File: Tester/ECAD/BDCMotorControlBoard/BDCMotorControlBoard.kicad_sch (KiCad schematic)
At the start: 45 parts, among them J3 SWIM connector, J4 Power connector, J5 Motor connector, J6 RS485 connector, Q1 2N7002, Q2 2N7002, Q7 2N7002, Q8 2N7002, SW1 SW_Push, U1 STM8S003F3P6, U3 SP485, U4 L78M05_TO252, Y1 Crystal_GND24

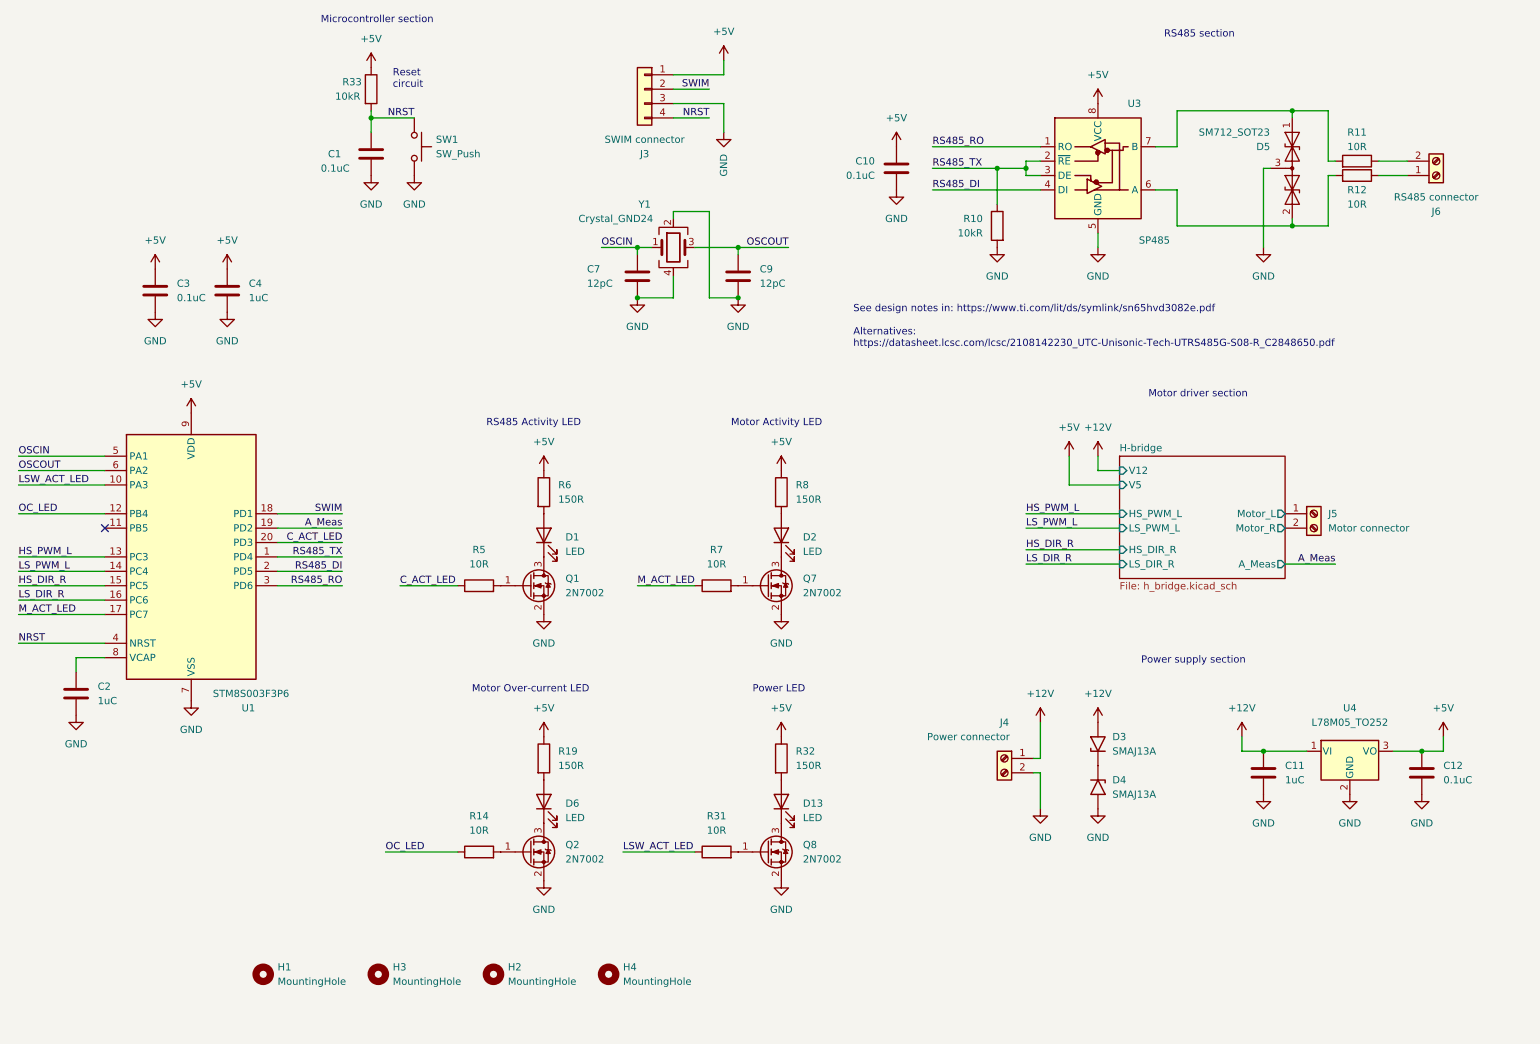
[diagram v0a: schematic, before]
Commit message: Progressed CAD
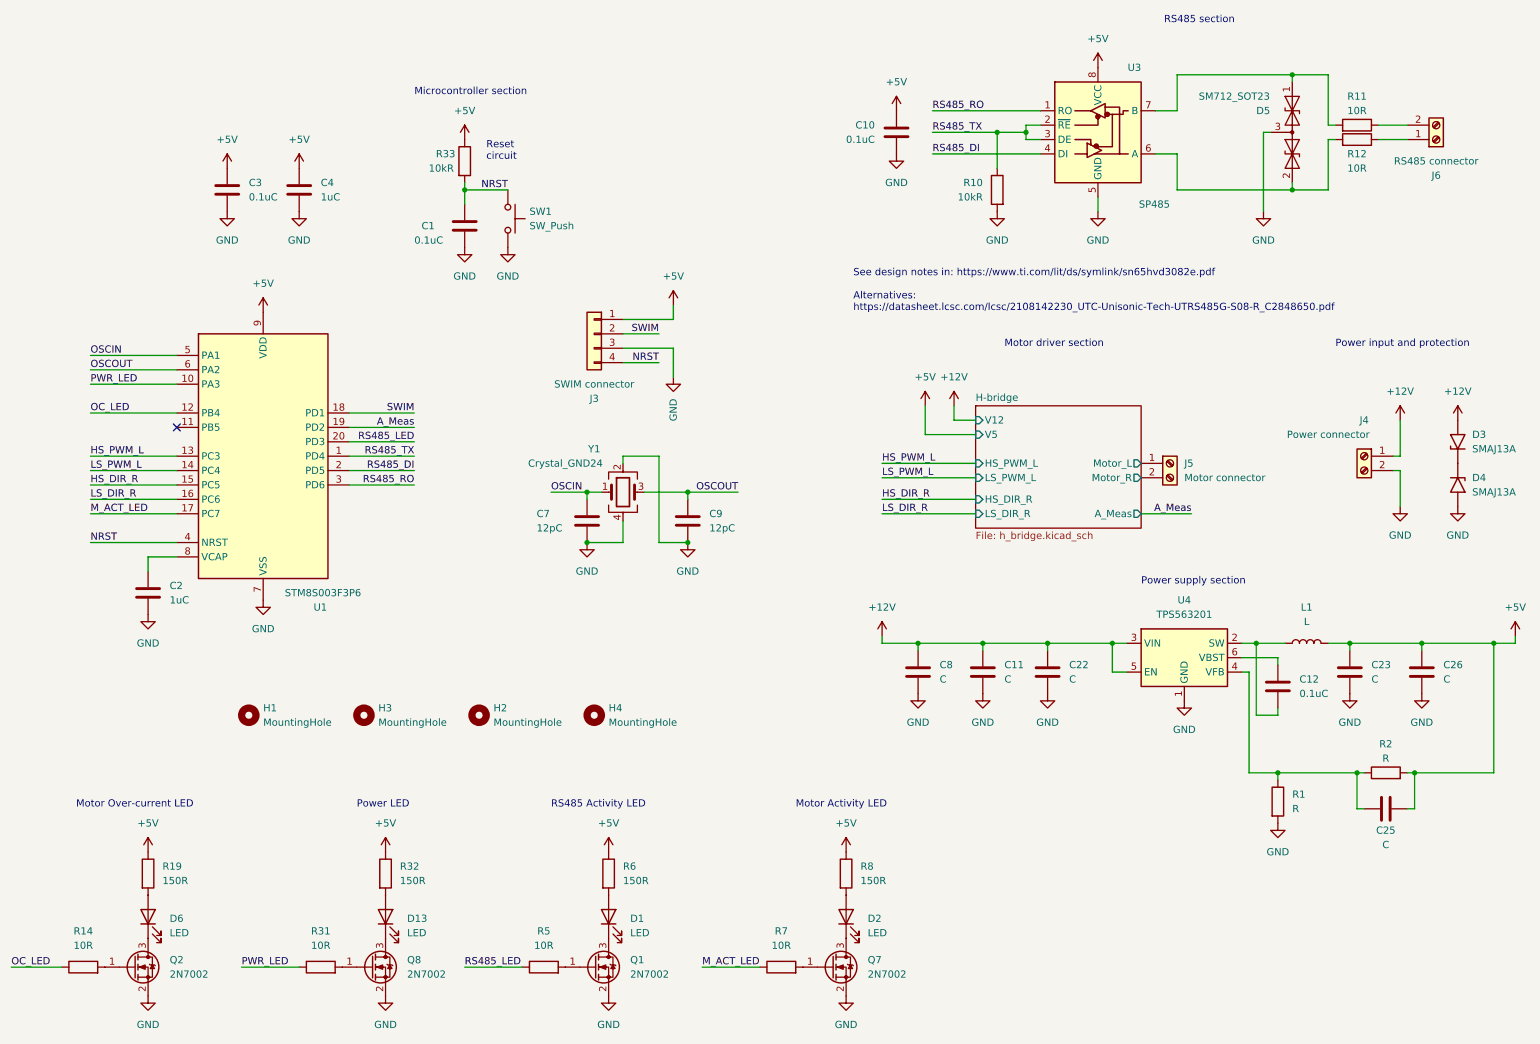
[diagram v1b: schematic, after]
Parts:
- removed U4: L78M05_TO252, Package_TO_SOT_SMD:TO-252-2, symbol Regulator_Linear:LM78M05_TO252
- added C22, C23, C25, C26, C8: C, symbol Device:C
- added L1: L, symbol Device:L
- added R1, R2: R, symbol Device:R
- added U4: TPS563201, Package_TO_SOT_SMD:SOT-23-6, symbol Regulator_Switching:TPS563200
- C11: value 1uC -> C; footprint Capacitor_SMD:C_0805_2012Metric_Pad1.18x1.45mm_HandSolder -> (none); Manufacturer Part Number GCM21BR71E105KA56L -> (none)
- H1, H2, H3, H4: Manufacturer Part Number (none) -> N/A
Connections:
- net +12V: now also C22.1, C8.1, U4.3 (VIN), U4.5 (EN)
- net +5V: now also C23.1, C25.2, C26.1, L1.2, R2.2; no longer C12.1
- net GND: now also C22.2, C23.2, C26.2, C8.2, R1.2, U4.1 (GND); no longer C12.2
- net C_ACT_LED renamed RS485_LED
- net LSW_ACT_LED renamed PWR_LED
- new net: C25.1, R1.1, R2.1, U4.4 (VFB)
- new net: C12.2, L1.1, U4.2 (SW)
- new net: C12.1, U4.6 (VBST)
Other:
- note added: "Power input and protection"
- moved on the sheet: C1, C10, C12, C2, C3, C4, C7, C9, D1, D13, D2, D3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
